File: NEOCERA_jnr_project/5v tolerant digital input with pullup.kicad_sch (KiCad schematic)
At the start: 11 parts, among them U15 74AHCT1G126, U17 74AHCT1G126, U19 74LCX244, U3 74AHCT1G126

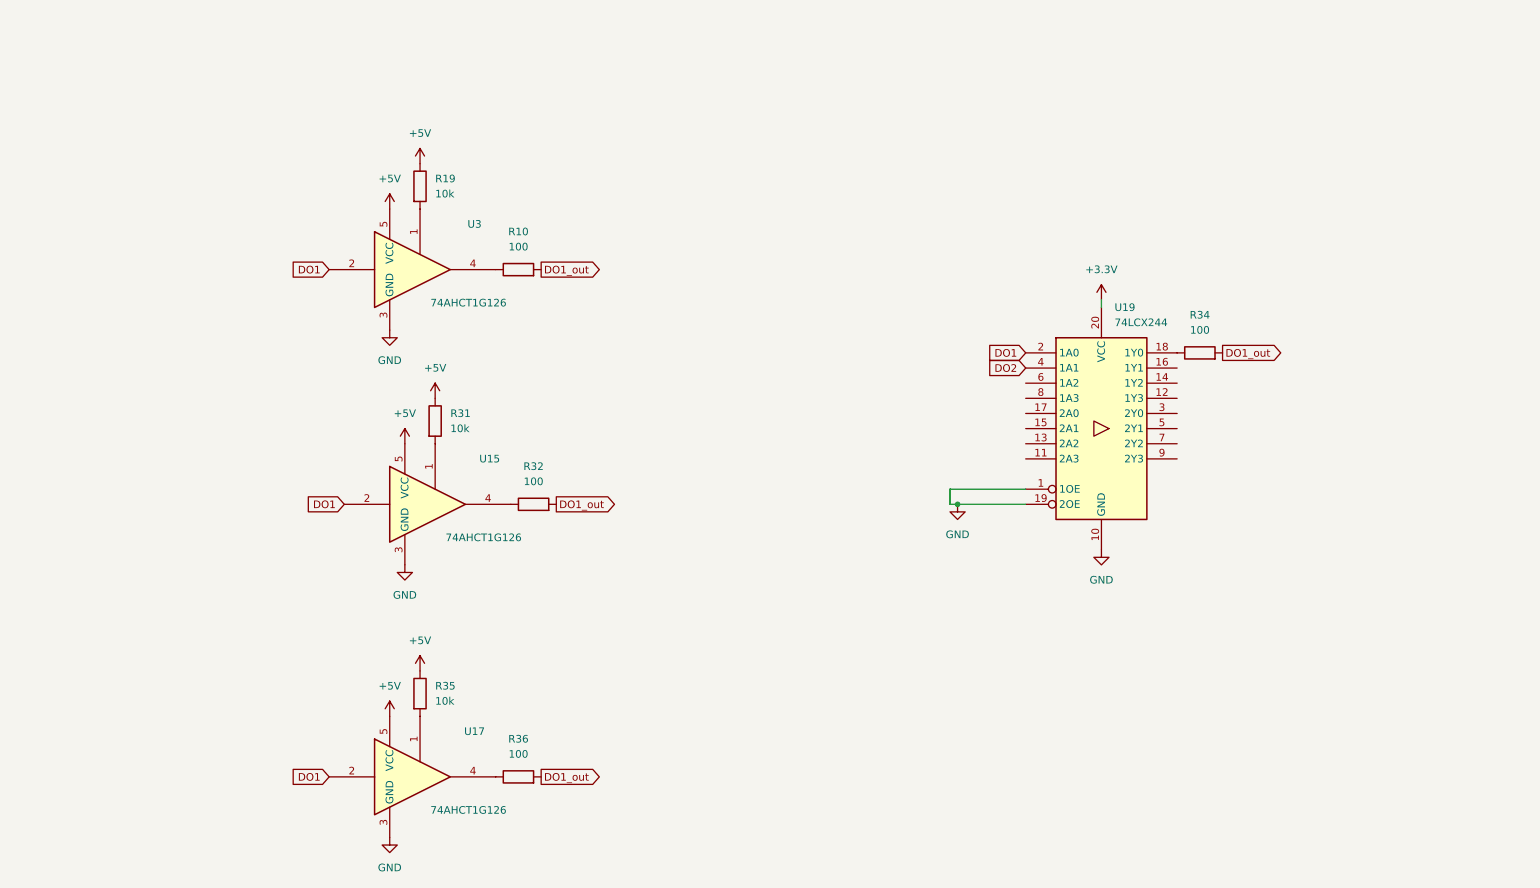
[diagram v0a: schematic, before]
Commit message: bunch of edits
bunch of edits were done including DB37
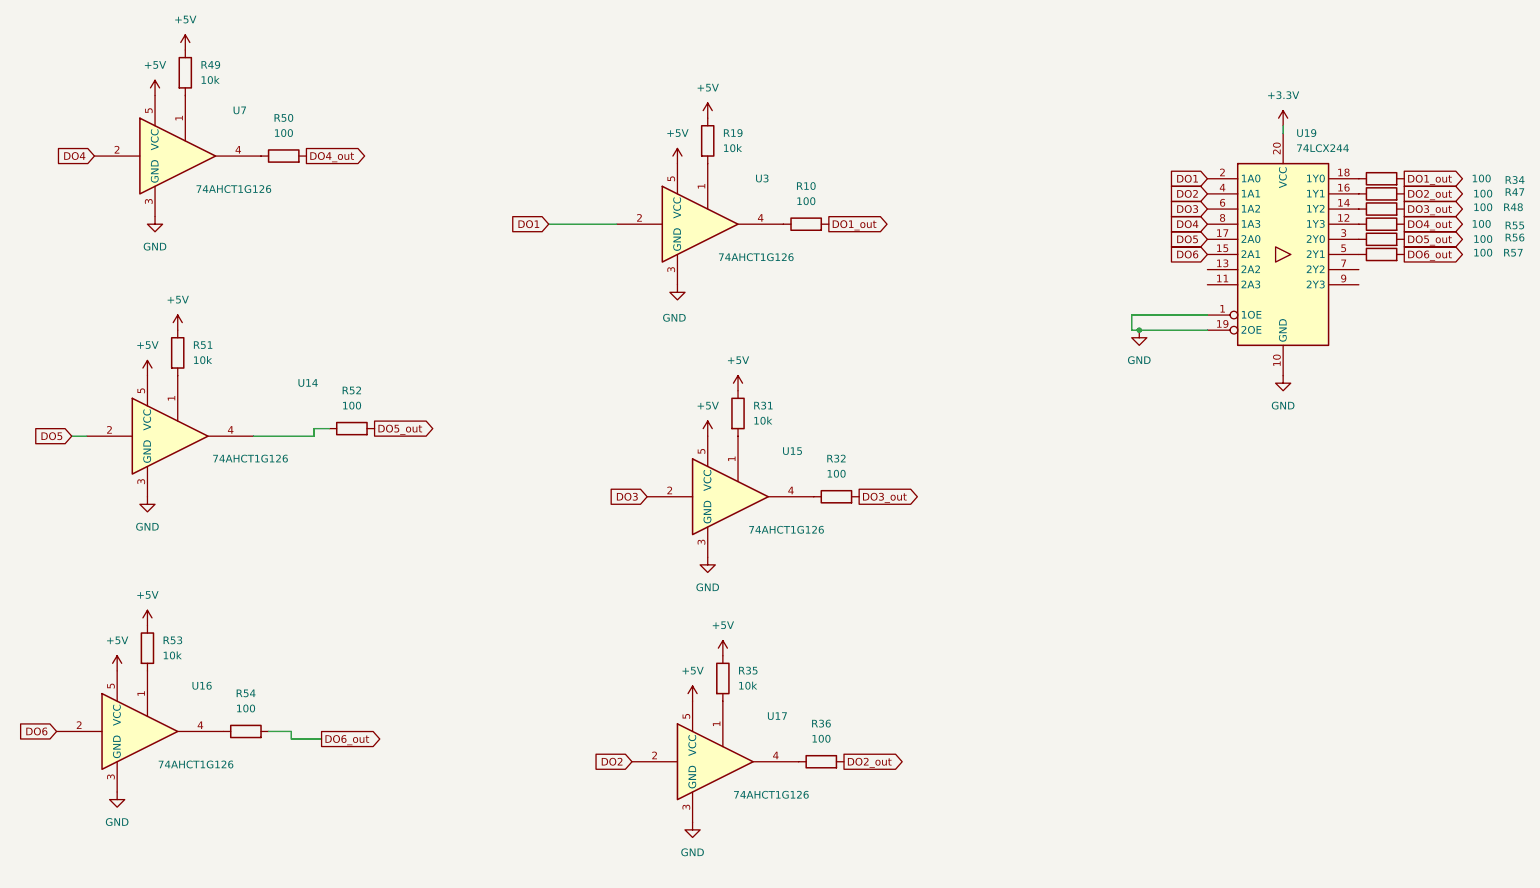
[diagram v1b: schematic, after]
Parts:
- added R47, R48, R50, R52, R54, R55, R56, R57: 100, Resistor_SMD:R_0603_1608Metric_Pad0.98x0.95mm_HandSolder, symbol Device:R
- added R49, R51, R53: 10k, Resistor_SMD:R_0603_1608Metric_Pad0.98x0.95mm_HandSolder, symbol Device:R
- added U14, U16, U7: 74AHCT1G126, Package_TO_SOT_SMD:SOT-23-5_HandSoldering, symbol 74xGxx:74AHCT1G126
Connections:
- net +5V: now also R49.1, R51.1, R53.1, U14.5 (VCC), U16.5 (VCC), U7.5 (VCC)
- net DO1: no longer U15.2, U17.2
- net DO1_out: no longer R32.2, R36.2
- net DO2: now also U17.2
- net GND: now also U14.3 (GND), U16.3 (GND), U7.3 (GND)
- net at U19.12 (1Y3): now also R55.1
- net at U19.14 (1Y2): now also R48.1
- net DO6: now reaches U19.15 (2A1)
- net DO6: now also U16.2
- net at U19.16 (1Y1): now also R47.1
- net DO5: now reaches U19.17 (2A0)
- net DO5: now also U14.2
- net at U19.3 (2Y0): now also R56.1
- net at U19.5 (2Y1): now also R57.1
- net DO3: now reaches U19.6 (1A2)
- net DO3: now also U15.2
- net DO4: now reaches U19.8 (1A3)
- net DO4: now also U7.2
- new net: R51.2, U14.1
- new net: R53.2, U16.1
- new net: R54.1, U16.4
- new net: R49.2, U7.1
- new net: R50.1, U7.4
- new net: R52.1, U14.4
- new net DO2_out: R36.2, R47.2
- new net DO3_out: R32.2, R48.2
- new net DO4_out: R50.2, R55.2
- new net DO5_out: R52.2, R56.2
- new net DO6_out: R54.2, R57.2
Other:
- moved on the sheet: R10, R19, R31, R32, R34, R35, R36, U15, U17, U19, U3
